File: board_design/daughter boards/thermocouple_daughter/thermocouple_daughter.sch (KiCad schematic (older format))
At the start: 10 parts, among them J1 Conn_01x09_Male, J2 Conn_01x02, U1 AD8613, U2 AD8495

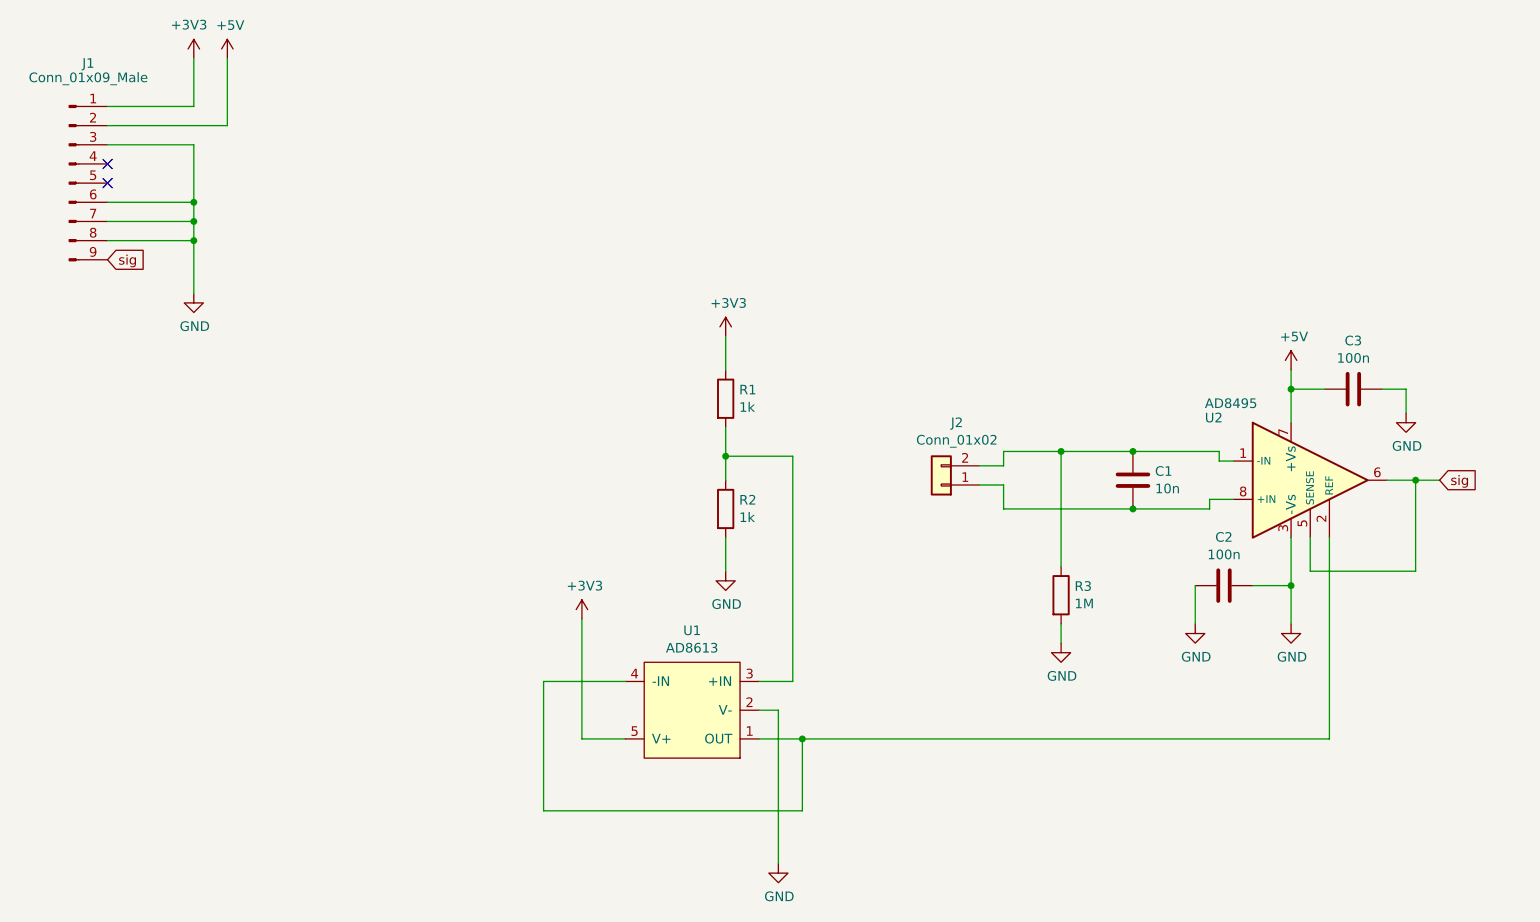
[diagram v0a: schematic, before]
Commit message: first MX export
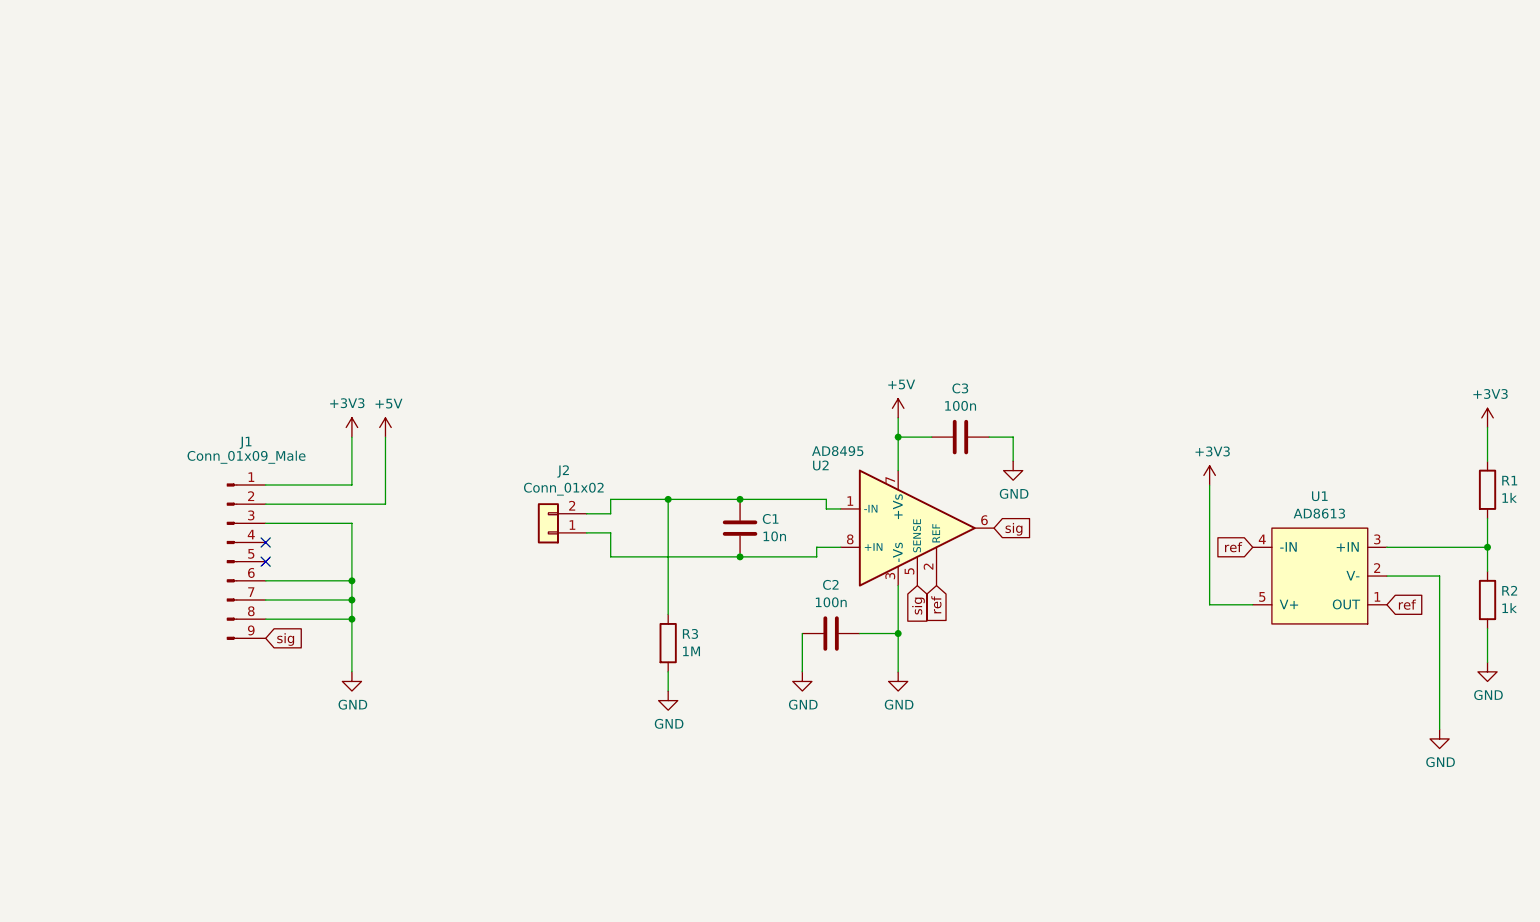
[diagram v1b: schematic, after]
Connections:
- net ref: now reaches U1.1 (OUT), U1.4 (-IN), U2.2 (REF)
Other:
- moved on the sheet: C1, C2, C3, J1, J2, R1, R2, R3, U1, U2
